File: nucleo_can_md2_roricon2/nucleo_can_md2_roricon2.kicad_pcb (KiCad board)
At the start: 2 copper layers, 63.7 x 58.6 mm, 24 parts, among them J1 Conn_01x05_Pin, J2 Conn_01x05_Pin, J3 Conn_01x02_Pin, U1 NUCLEO-F303K8, U2 MCP2562-E-P

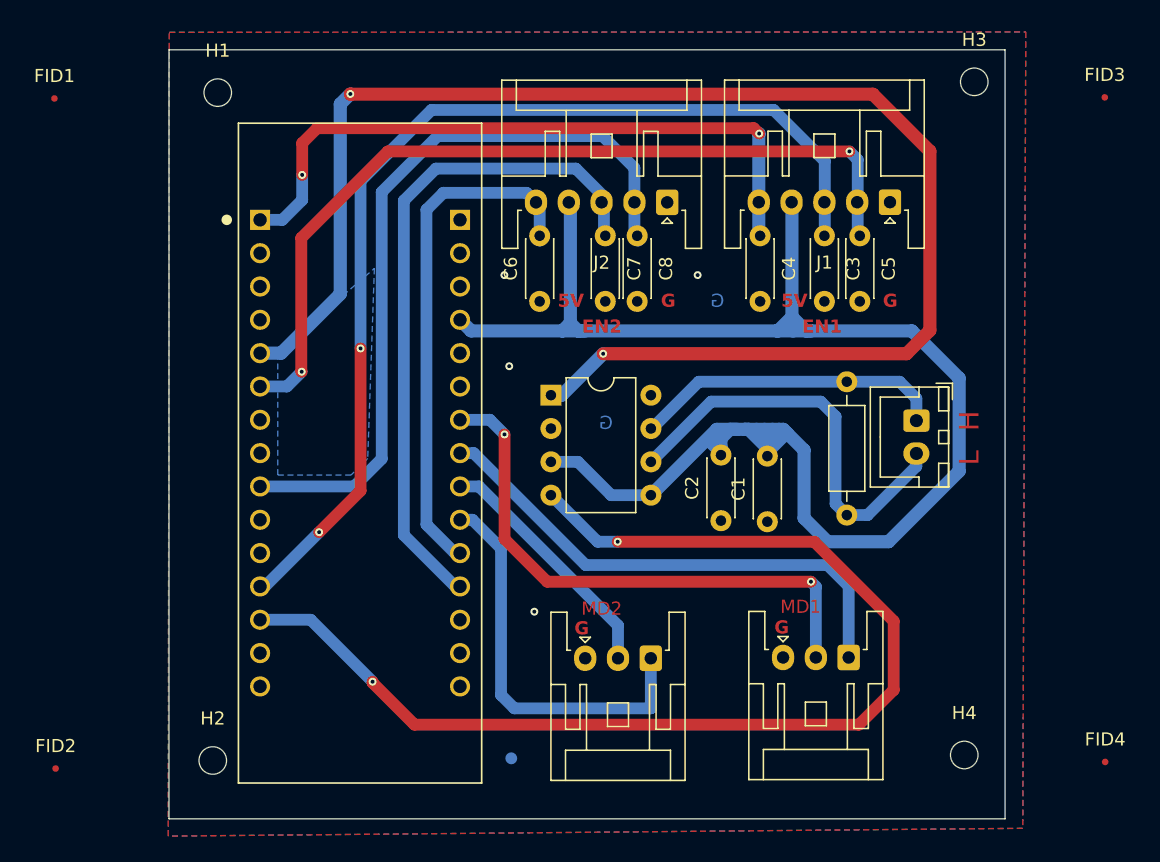
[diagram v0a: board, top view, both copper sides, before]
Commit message: 3.3v
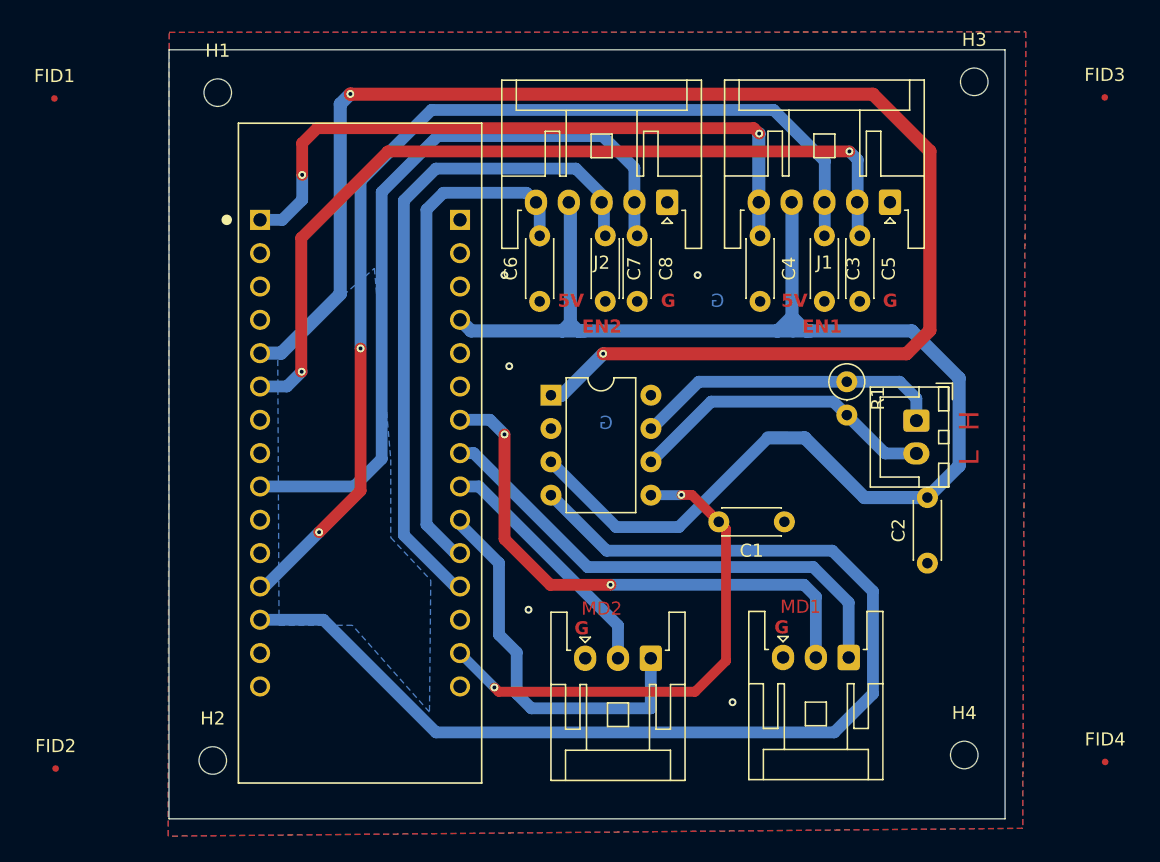
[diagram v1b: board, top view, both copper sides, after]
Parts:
- C1, C2, C3, C4, C5, C6, C7, C8: value 0.1μ -> 0.01μ
- R1: footprint Resistor_THT:R_Axial_DIN0207_L6.3mm_D2.5mm_P10.16mm_Horizontal -> Resistor_THT:R_Axial_DIN0207_L6.3mm_D2.5mm_P2.54mm_Vertical
- moved C2 16.1 mm to (172.4, 104.2)
- moved C1 1.30 mm to (161.6, 101.1), turned to 180 degrees
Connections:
- C1 pad 2: +5V -> +3.3V
- U1 pad 4_14: unconnected-(U1B-+3V3-Pad4_14) -> +3.3V
- U2 pad 5: +5V -> +3.3V
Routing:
- net +3.3V: track 0.00 -> 39.3 mm, vias 0 -> 2
- net +5V: track 126.6 -> 111.8 mm
- net /L: track 32.1 -> 23.8 mm
- net MD1_dir: track 30.6 -> 29.3 mm
- net CAN_Rx: track 88.1 -> 86.9 mm, vias 2 -> 0
- net MD2_dir: track 39.3 -> 38.5 mm
- net GND: track 0.33 -> 0.31 mm, vias 4 -> 5
